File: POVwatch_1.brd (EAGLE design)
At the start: 25.4 x 36.8 mm, 50 parts, among them Q1 S8050, U1 ATMEGA168P-AU, U2 ADXL345, U3 MCP6001-SOT23, U4 APDS-9008, U5 TP4056, U6 3.3V, Y1 7.3728MHz

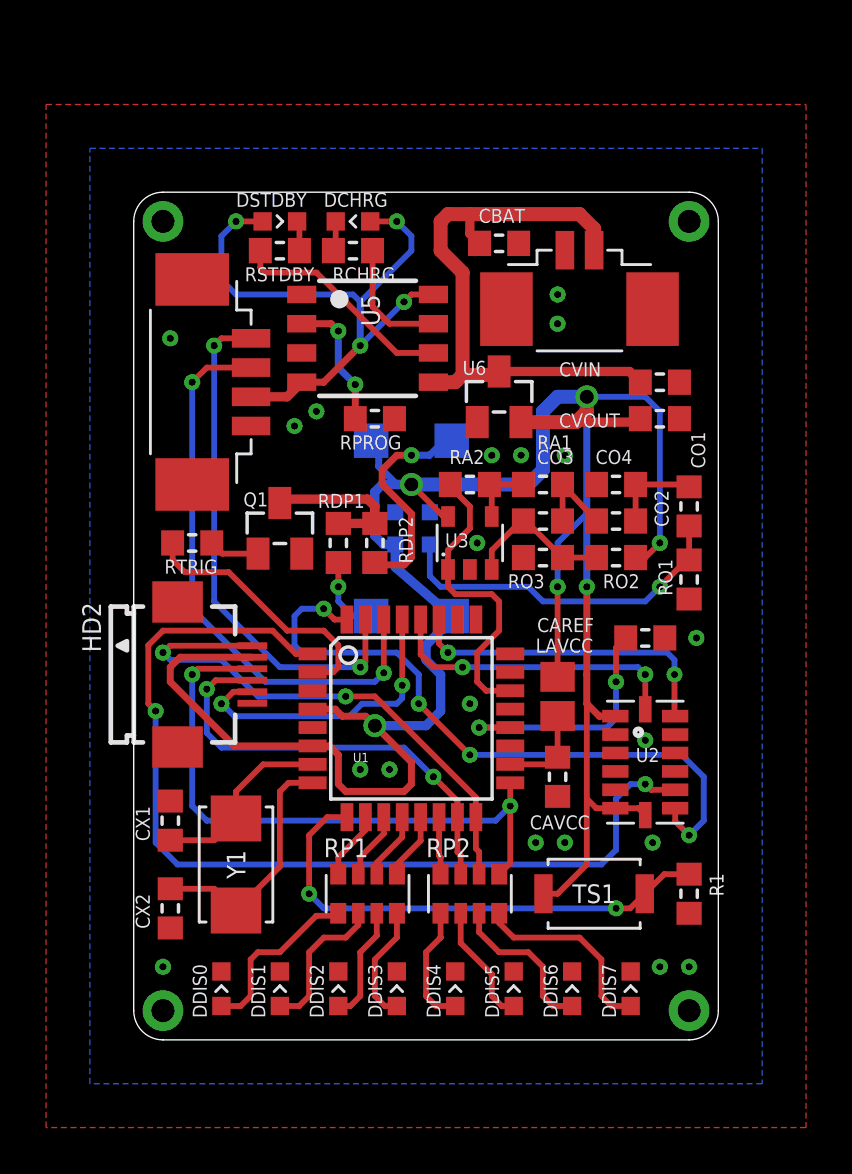
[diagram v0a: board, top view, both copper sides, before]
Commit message: This is POVwatch 1.1 (begin)
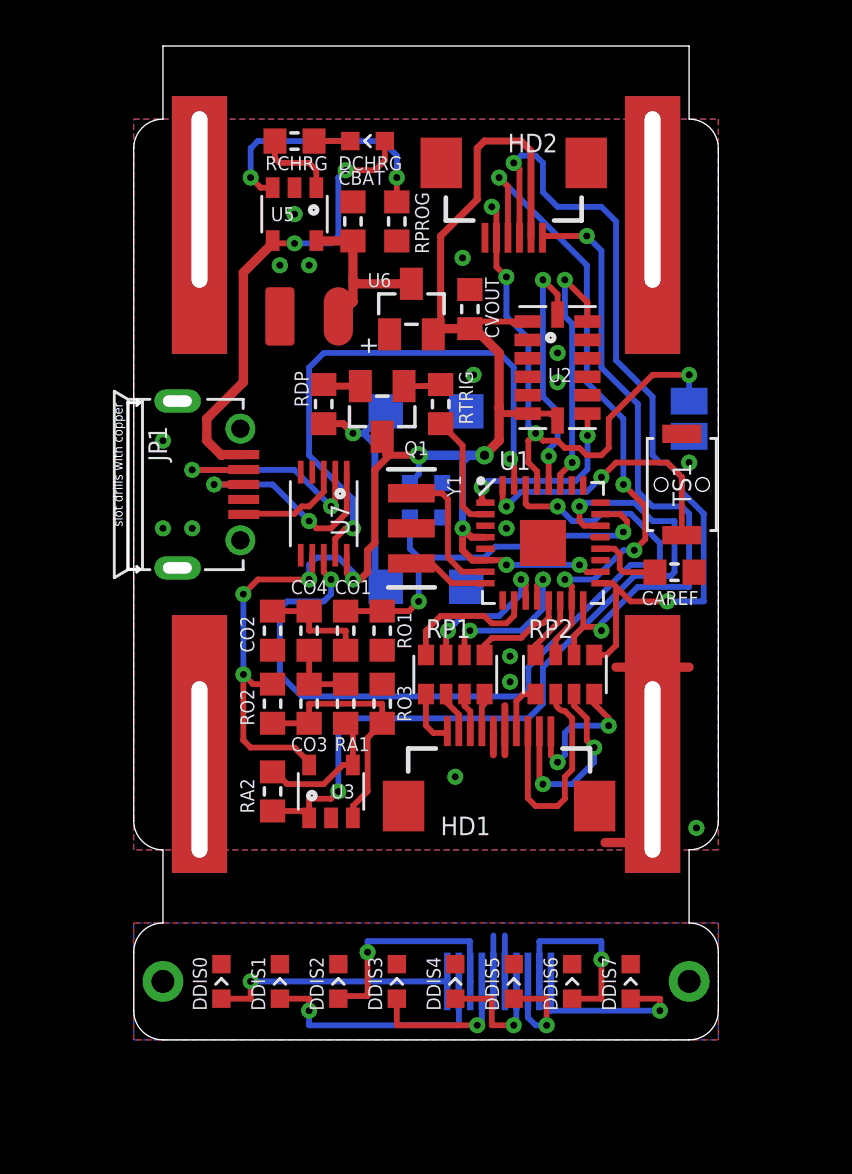
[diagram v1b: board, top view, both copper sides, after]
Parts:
- removed CAVCC: 100nF, MyLibrary:SMD0603
- removed CVIN: 1μF, MyLibrary:SMD0603
- removed CX1, CX2: 22pF, MyLibrary:SMD0603
- removed DSTDBY: GREEN, MyLibrary:LED-0603
- removed LAVCC: 22μH, MyLibrary:SMD0805
- removed R1: 10kΩ, MyLibrary:SMD0603
- removed RDP1, RDP2: 220Ω, MyLibrary:SMD0603
- removed RSTDBY: 1kΩ, MyLibrary:SMD0603
- added FB1, FB2, FB3, FB4: BROAD-STICK, MyLibrary:BOARD-STICK
- added HD3: HEADER1X10, MyLibrary:FPC0.5-10-SOLDER
- added JP1: USB-MICRO, MyLibrary:USB-MICRO-5+6P-SMD-0.65-AB
- added RDP: 220Ω, MyLibrary:SMD0603
- added RESET: JUMPER-SMD, MyLibrary:JMPER-SMD
- added U$1: (no value), MyLibrary:ICON-CE
- added U$2: (no value), MyLibrary:ICON-PW
- added U7: CH340E, MyLibrary:MSOP10
- HD1: value HEADER1X4-SMD1.25 -> HEADER1X10-FPC0.5; device MyLibrary:SMD1.25-1X4 -> MyLibrary:FPC0.5-10
- LI-ION: value BATTERY-SMD1.25 -> BATTERY-SMD; device MyLibrary:SMD1.25-1X2 -> MyLibrary:BAT-SMD
- TS1: value TS-3035 -> TS-P; device MyLibrary:TS-3X4 -> MyLibrary:TS-3X4P
- U1: value ATMEGA168P-AU -> ATMEGA168P-QFN32; device MyLibrary:TQFP32 -> MyLibrary:QFN32
- U5: value TP4056 -> TP4055; device MyLibrary:SOP8 -> MyLibrary:SOT23-5
- Y1: device MyLibrary:XTAL-5032 -> MyLibrary:CSTCE
- moved HD2 26.6 mm to (16.5, 38.1), turned to 180 degrees
- moved HD1 20.8 mm to (15.9, 10.2), turned to 0 degrees
- moved TS1 18.2 mm to (23.8, 24.1), turned to 90 degrees
- moved U2 17.6 mm to (18.4, 29.2)
- moved Y1 16.5 mm to (12.1, 22.2)
- moved CO4 16.2 mm to (6.03, 17.8), turned to 270 degrees
- moved RO2 16.2 mm to (6.03, 14.6), turned to 90 degrees
- moved CO1 15.9 mm to (9.21, 17.8), turned to 90 degrees
- moved RA2 15.9 mm to (6.03, 10.8), turned to 90 degrees
- moved CO2 14.2 mm to (7.62, 17.8), turned to 90 degrees
- moved RO1 13.5 mm to (10.8, 17.8)
- moved CO3 12.9 mm to (7.62, 14.6), turned to 90 degrees
- moved RA1 12.8 mm to (9.21, 14.6), turned to 90 degrees
- moved LI-ION 12.7 mm to (7.62, 31.4), turned to 0 degrees
- moved RTRIG 12.4 mm to (13.3, 27.6), turned to 270 degrees
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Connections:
- net CHRGR renamed DRCHRG
- net TRIGR renamed RQTRIG
- removed net AVCC: CAVCC.2, LAVCC.1, U1.18
- removed net BUTTON: R1.1, TS1.2, U1.9
- removed net CHRG: RCHRG.1, U5.7
- removed net COLLECT: Q1.3, RDP1.1, RDP2.1
- removed net INT2: U1.1, U2.9
- removed net LR1: DP1.C, RDP1.2
- removed net LR2: DP2.C, RDP2.2
- removed net N$22: DDIS1.A, RP1.4
- removed net N$23: DDIS2.A, RP1.6
- removed net N$24: DDIS3.A, RP1.8
- removed net N$25: DDIS4.A, RP2.2
- removed net N$26: DDIS5.A, RP2.4
- removed net N$27: DDIS6.A, RP2.6
- removed net N$28: DDIS7.A, RP2.8
- removed net N$29: DDIS0.A, RP1.2
- removed net PROGR: RPROG.1, U5.2
- removed net STDBY: RSTDBY.1, U5.6
- removed net STDBYR: DSTDBY.C, RSTDBY.2
- removed net VCC: DCHRG.A, DSTDBY.A, HD1.2, U5.4, U5.8
- new net !CHRG: RCHRG.1, U5.1
- new net !GND: DDIS0.C, DDIS1.C, DDIS2.C, DDIS3.C, DDIS4.C, DDIS5.C, DDIS6.C, DDIS7.C, HD3.5, HD3.6
- new net GND(CH340E): JP1.5, U7.3
- new net HD0: DDIS0.A, HD3.1
- new net HD1: DDIS1.A, HD3.2
- new net HD2: DDIS2.A, HD3.3
- new net HD3: DDIS3.A, HD3.4
- new net HD4: DDIS4.A, HD3.7
- new net HD5: DDIS5.A, HD3.8
- new net HD6: DDIS6.A, HD3.9
- new net HD7: DDIS7.A, HD3.10
- new net INT0: TS1.1, U1.32
- new net PROG: RPROG.1, U5.3
- new net QRP: Q1.2, RDP.2
- new net RDP: DP1.A, DP2.A, RDP.1
- new net RH0: HD1.1, RP1.2
- new net RH1: HD1.2, RP1.4
- new net RH2: HD1.3, RP1.6
- new net RH3: HD1.4, RP1.8
- new net RH4: HD1.7, RP2.2
- new net RH5: HD1.8, RP2.4
- new net RH6: HD1.9, RP2.6
- new net RH7: HD1.10, RP2.8
- new net UD+: JP1.3, U7.1
- new net UD-: JP1.2, U7.2
- new net VUSB: DCHRG.A, JP1.1, U5.4
- net GND: now also DP1.C, DP2.C, FB1.BOT, FB1.TOP, FB2.BOT, FB2.TOP, FB3.BOT, FB3.TOP, FB4.BOT, FB4.TOP, HD1.5, HD1.6, JP1.P1, JP1.P2, JP1.P3, JP1.P4, LI-ION.-, RESET.1, TS1.2, U1.EP, U5.2, Y1.2; no longer CAVCC.1, CVIN.2, CX1.1, CX2.1, DDIS0.C, DDIS1.C, DDIS2.C, DDIS3.C, DDIS4.C, DDIS5.C, DDIS6.C, DDIS7.C, HD1.1, LI-ION.2, Q1.2, R1.2, U5.1, U5.3
- net INT1: now also U1.1; no longer U1.32
- net OUT0: now also U1.23
- net RESET: now also RESET.2
- net RXD: now also U7.8; no longer HD1.3
- net TXD: now also U7.9; no longer HD1.4
- net VBAT: now also LI-ION.+; no longer CVIN.1, LI-ION.1
- net VDD_3V3: now also Q1.3, U1.18, U7.10, U7.7; no longer DP1.A, DP2.A, LAVCC.2, TS1.1
- net X1: no longer CX1.2
- net X2: now also Y1.3; no longer CX2.2, Y1.2
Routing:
- net INT2: track 42.3 -> 0.00 mm, vias 2 -> 0
- net VDD_3V3: track 112.3 -> 74.2 mm, vias 6 -> 9
- net VCC: track 27.9 -> 0.00 mm, vias 4 -> 0
- net BUTTON: track 21.9 -> 0.00 mm, vias 2 -> 0
- net INT1: track 29.0 -> 8.07 mm, vias 4 -> 2
- net VUSB: track 0.00 -> 20.5 mm, vias 0 -> 2
- net PULSE: track 13.4 -> 33.3 mm, vias 0 -> 2
- net VBAT: track 25.9 -> 7.75 mm
- net INT0: track 0.00 -> 12.2 mm, vias 0 -> 2
- net PROG: track 0.00 -> 11.2 mm, vias 0 -> 2
- net HD1: track 0.00 -> 10.8 mm, vias 0 -> 1
- net RXD: track 24.8 -> 35.5 mm
- net HD0: track 0.00 -> 10.6 mm, vias 0 -> 1
- net UD-: track 0.00 -> 10.5 mm, vias 0 -> 2
- net RDP: track 0.00 -> 10.3 mm, vias 0 -> 1
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- added copper zone on layer 1, net !GND
- added copper zone on layer 16, net !GND
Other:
- board size 25.4 x 36.8 mm -> 25.4 x 43.2 mm
- board text added: "Ver 1.1"
- board text removed: "Design by geneLocated"
- board text removed: "Devised & Assembled in China"
- board text removed: "POVwatch"
- board text removed: "Ver 1.0"
